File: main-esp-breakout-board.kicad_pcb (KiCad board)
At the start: 2 copper layers, 170.5 x 109 mm, 3 parts, among them J2 Conn_01x18_Pin, J3 Conn_01x18_Pin

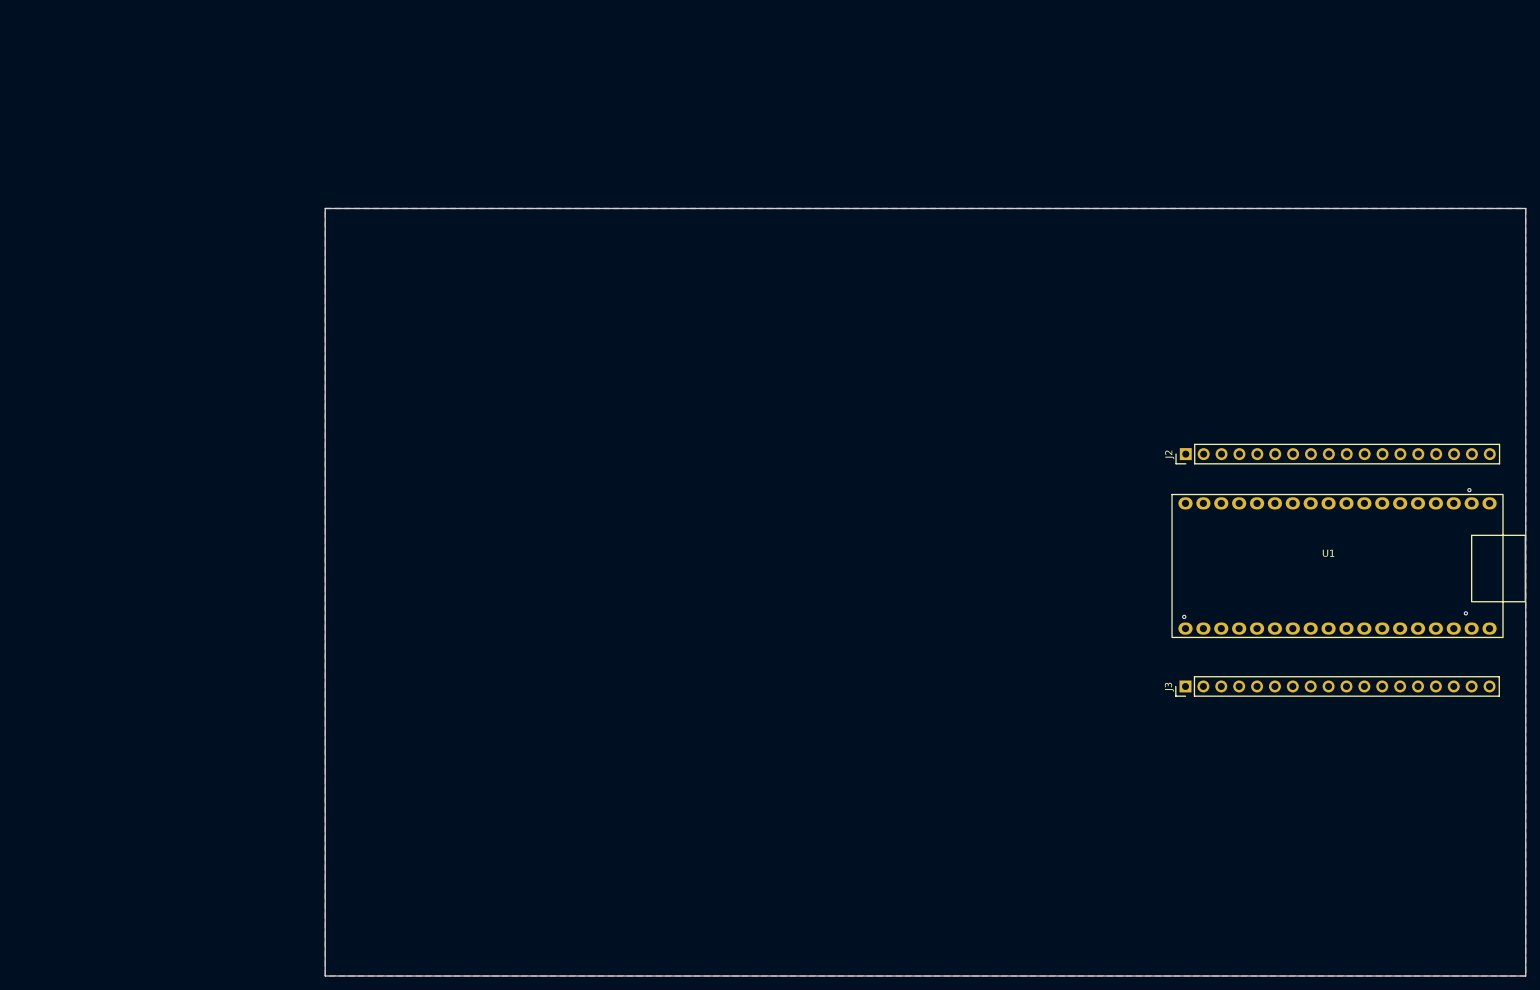
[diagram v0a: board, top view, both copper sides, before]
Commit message: halfway thru layout...
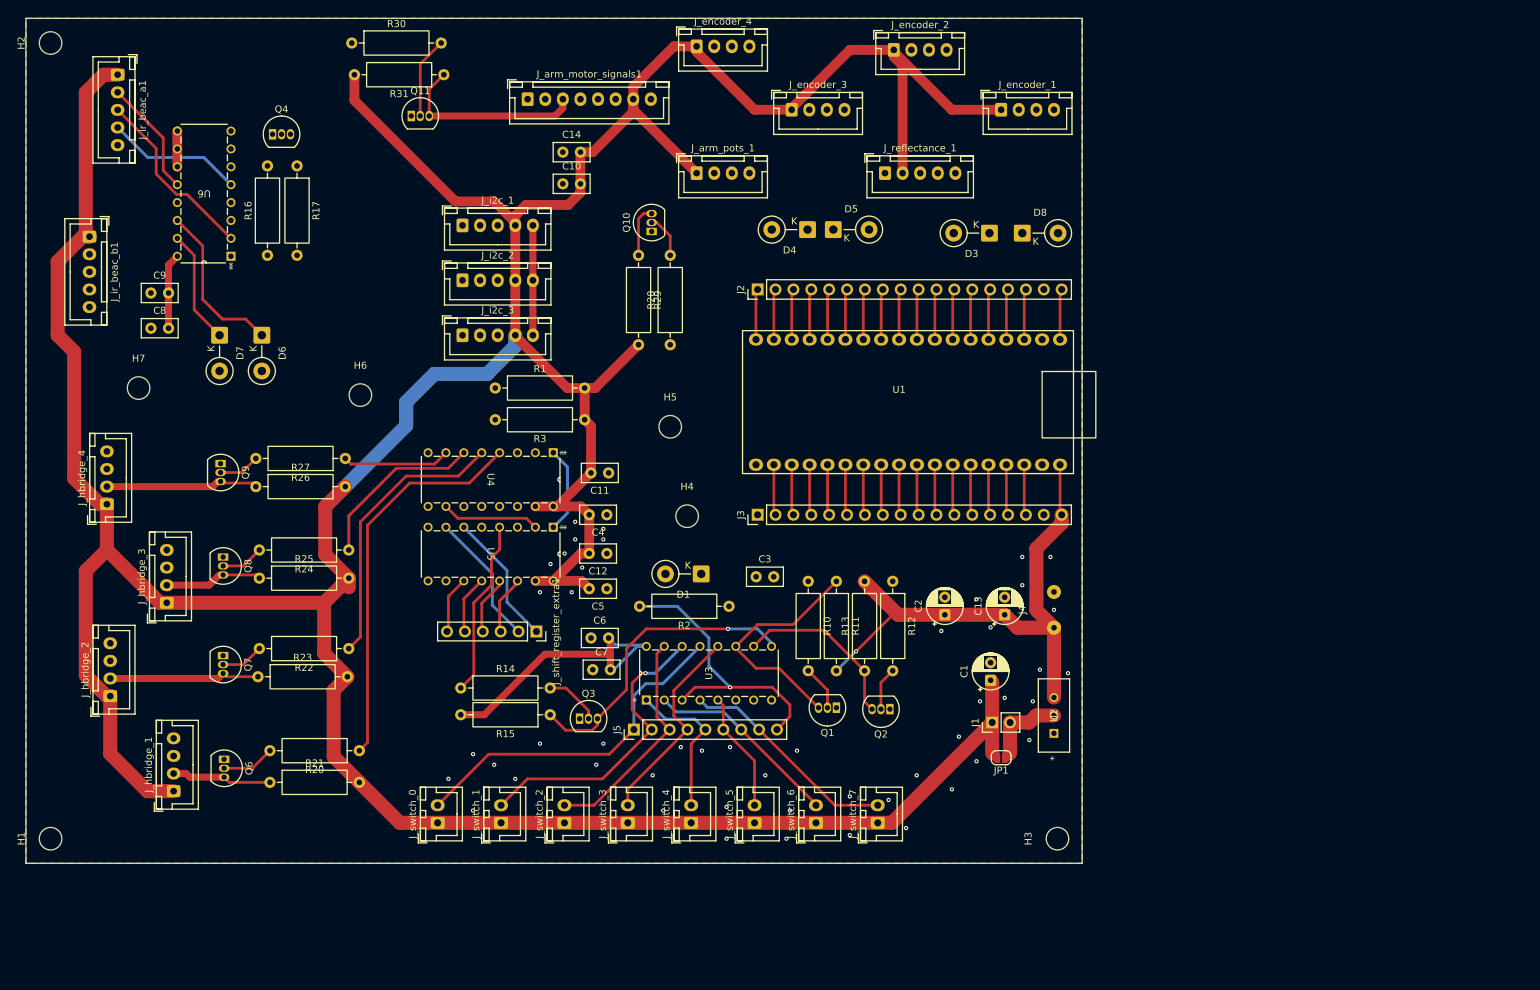
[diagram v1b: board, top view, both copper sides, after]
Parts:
- added C1: 10uf, Capacitor_THT:CP_Radial_D5.0mm_P2.50mm, F.Cu at (149.5, 106.5)
- added C10: 1nF, Capacitor_THT:C_Disc_D5.0mm_W2.5mm_P2.50mm, F.Cu at (88.8, 36.0)
- added C11: 1nF, Capacitor_THT:C_Disc_D5.0mm_W2.5mm_P2.50mm, F.Cu at (95.2, 77.1)
- added C12: 1nF, Capacitor_THT:C_Disc_D5.0mm_W2.5mm_P2.50mm, F.Cu at (95.0, 88.5)
- added C13: 10uf, Capacitor_THT:CP_Radial_D5.0mm_P2.50mm, F.Cu at (151.5, 97.2)
- added C14: 1nF, Capacitor_THT:C_Disc_D5.0mm_W2.5mm_P2.50mm, F.Cu at (88.8, 31.5)
- added C2: 1uf, Capacitor_THT:CP_Radial_D5.0mm_P2.50mm, F.Cu at (143.0, 97.2)
- added C3: 100nF, Capacitor_THT:C_Disc_D5.0mm_W2.5mm_P2.50mm, F.Cu at (116.2, 91.8)
- added C4: 1nF, Capacitor_THT:C_Disc_D5.0mm_W2.5mm_P2.50mm, F.Cu at (95.0, 83.0)
- added C5: 1nF, Capacitor_THT:C_Disc_D5.0mm_W2.5mm_P2.50mm, F.Cu at (95.0, 93.5)
- added C6: 1nF, Capacitor_THT:C_Disc_D5.0mm_W2.5mm_P2.50mm, F.Cu at (92.8, 100.5)
- added C7: 1nF, Capacitor_THT:C_Disc_D5.0mm_W2.5mm_P2.50mm, F.Cu at (93.0, 105.0)
- added C8: 1nF, Capacitor_THT:C_Disc_D5.0mm_W2.5mm_P2.50mm, F.Cu at (30.2, 56.5)
- added C9: 1nF, Capacitor_THT:C_Disc_D5.0mm_W2.5mm_P2.50mm, F.Cu at (30.2, 51.5)
- added D1: 3V3, Diode_THT:D_DO-15_P5.08mm_Vertical_KathodeUp, F.Cu at (108.4, 91.4)
- added D3: 3V3, Diode_THT:D_DO-15_P5.08mm_Vertical_KathodeUp, F.Cu at (149.3, 43.0)
- added D4: 3V3, Diode_THT:D_DO-15_P5.08mm_Vertical_KathodeUp, F.Cu at (123.5, 42.5)
- added D5: 3V3, Diode_THT:D_DO-15_P5.08mm_Vertical_KathodeUp, F.Cu at (127.2, 42.5)
- added D6: 3V3, Diode_THT:D_DO-15_P5.08mm_Vertical_KathodeUp, F.Cu at (46.0, 57.5)
- added D7: 3V3, Diode_THT:D_DO-15_P5.08mm_Vertical_KathodeUp, F.Cu at (40.0, 57.5)
- added D8: 3V3, Diode_THT:D_DO-15_P5.08mm_Vertical_KathodeUp, F.Cu at (154.0, 43.0)
- added H1: MountingHole, MountingHole:MountingHole_3.2mm_M3, F.Cu at (16.0, 129.0)
- added H2: MountingHole, MountingHole:MountingHole_3.2mm_M3, F.Cu at (16.0, 16.0)
- added H3: MountingHole, MountingHole:MountingHole_3.2mm_M3, F.Cu at (159.0, 129.0)
- added H4: MountingHole, MountingHole:MountingHole_3.2mm_M3, F.Cu at (106.4, 83.2)
- added H5: MountingHole, MountingHole:MountingHole_3.2mm_M3, F.Cu at (104.0, 70.5)
- added H6: MountingHole, MountingHole:MountingHole_3.2mm_M3, F.Cu at (60.0, 66.0)
- added H7: MountingHole, MountingHole:MountingHole_3.2mm_M3, F.Cu at (28.5, 65.0)
- added J1: Conn_01x02_Pin, Connector_PinHeader_2.54mm:PinHeader_1x02_P2.54mm_Vertical, F.Cu at (149.7, 112.5)
- added J4: Conn_01x02_Socket, Project_Lib:Power_Connector, F.Cu at (158.5, 96.5)
- added J5: Conn_01x09_Pin, Connector_PinHeader_2.54mm:PinHeader_1x09_P2.54mm_Vertical, F.Cu at (98.8, 113.5)
- added JP1: SolderJumper_2_Open, Jumper:SolderJumper-2_P1.3mm_Open_RoundedPad1.0x1.5mm, F.Cu at (151.0, 117.5)
- added J_arm_motor_signals1: Conn_01x08_Socket, Connector_JST:JST_XH_B8B-XH-A_1x08_P2.50mm_Vertical, F.Cu at (83.8, 24.0)
- added J_arm_pots_1: Conn_01x04_Socket, Connector_JST:JST_XH_B4B-XH-A_1x04_P2.50mm_Vertical, F.Cu at (107.8, 34.5)
- added J_encoder_1: Conn_01x04_Socket, Connector_JST:JST_XH_B4B-XH-A_1x04_P2.50mm_Vertical, F.Cu at (151.0, 25.5)
- added J_encoder_2: Conn_01x04_Socket, Connector_JST:JST_XH_B4B-XH-A_1x04_P2.50mm_Vertical, F.Cu at (135.8, 17.0)
- added J_encoder_3: Conn_01x04_Socket, Connector_JST:JST_XH_B4B-XH-A_1x04_P2.50mm_Vertical, F.Cu at (121.2, 25.5)
- added J_encoder_4: Conn_01x04_Socket, Connector_JST:JST_XH_B4B-XH-A_1x04_P2.50mm_Vertical, F.Cu at (107.8, 16.5)
- added J_hbridge_1: Conn_01x04_Socket, Connector_JST:JST_XH_B4B-XH-A_1x04_P2.50mm_Vertical, F.Cu at (33.5, 122.2)
- added J_hbridge_2: Conn_01x04_Socket, Connector_JST:JST_XH_B4B-XH-A_1x04_P2.50mm_Vertical, F.Cu at (24.5, 108.8)
- added J_hbridge_3: Conn_01x04_Socket, Connector_JST:JST_XH_B4B-XH-A_1x04_P2.50mm_Vertical, F.Cu at (32.5, 95.5)
- added J_hbridge_4: Conn_01x04_Socket, Connector_JST:JST_XH_B4B-XH-A_1x04_P2.50mm_Vertical, F.Cu at (24.0, 81.5)
- added J_i2c_1: Conn_01x05_Socket, Connector_JST:JST_XH_B5B-XH-A_1x05_P2.50mm_Vertical, F.Cu at (74.5, 41.9)
- added J_i2c_2: Conn_01x05_Socket, Connector_JST:JST_XH_B5B-XH-A_1x05_P2.50mm_Vertical, F.Cu at (74.5, 49.7)
- added J_i2c_3: Conn_01x05_Socket, Connector_JST:JST_XH_B5B-XH-A_1x05_P2.50mm_Vertical, F.Cu at (74.5, 57.5)
- added J_ir_beac_a1: Conn_01x05_Socket, Connector_JST:JST_XH_B5B-XH-A_1x05_P2.50mm_Vertical, F.Cu at (25.5, 20.5)
- added J_ir_beac_b1: Conn_01x05_Socket, Connector_JST:JST_XH_B5B-XH-A_1x05_P2.50mm_Vertical, F.Cu at (21.5, 43.5)
- added J_reflectance_1: Conn_01x05_Socket, Connector_JST:JST_XH_B5B-XH-A_1x05_P2.50mm_Vertical, F.Cu at (134.5, 34.5)
- added J_shift_register_extra1: Conn_01x06_Pin, Connector_PinSocket_2.54mm:PinSocket_1x06_P2.54mm_Vertical, F.Cu at (85.0, 99.6)
- added J_switch_0: Conn_01x02_Socket, Connector_JST:JST_XH_B2B-XH-A_1x02_P2.50mm_Vertical, F.Cu at (71.0, 126.8)
- added J_switch_1: Conn_01x02_Socket, Connector_JST:JST_XH_B2B-XH-A_1x02_P2.50mm_Vertical, F.Cu at (80.0, 126.8)
- added J_switch_2: Conn_01x02_Socket, Connector_JST:JST_XH_B2B-XH-A_1x02_P2.50mm_Vertical, F.Cu at (89.0, 126.8)
- added J_switch_3: Conn_01x02_Socket, Connector_JST:JST_XH_B2B-XH-A_1x02_P2.50mm_Vertical, F.Cu at (98.0, 126.8)
- added J_switch_4: Conn_01x02_Socket, Connector_JST:JST_XH_B2B-XH-A_1x02_P2.50mm_Vertical, F.Cu at (107.0, 126.8)
- added J_switch_5: Conn_01x02_Socket, Connector_JST:JST_XH_B2B-XH-A_1x02_P2.50mm_Vertical, F.Cu at (116.0, 126.8)
- added J_switch_6: Conn_01x02_Socket, Connector_JST:JST_XH_B2B-XH-A_1x02_P2.50mm_Vertical, F.Cu at (124.7, 126.8)
- added J_switch_7: Conn_01x02_Socket, Connector_JST:JST_XH_B2B-XH-A_1x02_P2.50mm_Vertical, F.Cu at (133.5, 126.8)
- added Q1: 2N3904, Package_TO_SOT_THT:TO-92_Inline, F.Cu at (127.6, 110.4)
- added Q10: 2N3904, Package_TO_SOT_THT:TO-92_Inline, F.Cu at (101.4, 42.8)
- added Q11: 2N3904, Package_TO_SOT_THT:TO-92_Inline, F.Cu at (67.2, 26.4)
- added Q2: 2N3904, Package_TO_SOT_THT:TO-92_Inline, F.Cu at (135.2, 110.6)
- added Q3: 2N3904, Package_TO_SOT_THT:TO-92_Inline, F.Cu at (91.1, 112.0)
- added Q4: 2N3904, Package_TO_SOT_THT:TO-92_Inline, F.Cu at (47.5, 29.0)
- added Q6: 2N3904, Package_TO_SOT_THT:TO-92_Inline, F.Cu at (40.6, 117.7)
- added Q7: 2N3904, Package_TO_SOT_THT:TO-92_Inline, F.Cu at (40.5, 103.0)
- added Q8: 2N3904, Package_TO_SOT_THT:TO-92_Inline, F.Cu at (40.5, 89.0)
- added Q9: 2N3904, Package_TO_SOT_THT:TO-92_Inline, F.Cu at (40.1, 75.7)
- added R1: 4.7k, Resistor_THT:R_Axial_DIN0309_L9.0mm_D3.2mm_P12.70mm_Horizontal, F.Cu at (79.2, 65.0)
- added R10: 100k, Resistor_THT:R_Axial_DIN0309_L9.0mm_D3.2mm_P12.70mm_Horizontal, F.Cu at (123.6, 92.5)
- added R11: 10k, Resistor_THT:R_Axial_DIN0309_L9.0mm_D3.2mm_P12.70mm_Horizontal, F.Cu at (127.6, 92.5)
- added R12: 100k, Resistor_THT:R_Axial_DIN0309_L9.0mm_D3.2mm_P12.70mm_Horizontal, F.Cu at (135.6, 92.5)
- added R13: 10k, Resistor_THT:R_Axial_DIN0309_L9.0mm_D3.2mm_P12.70mm_Horizontal, F.Cu at (131.6, 105.2)
- added R14: 100k, Resistor_THT:R_Axial_DIN0309_L9.0mm_D3.2mm_P12.70mm_Horizontal, F.Cu at (74.2, 107.6)
- added R15: 10k, Resistor_THT:R_Axial_DIN0309_L9.0mm_D3.2mm_P12.70mm_Horizontal, F.Cu at (87.0, 111.4)
- added R16: 100k, Resistor_THT:R_Axial_DIN0309_L9.0mm_D3.2mm_P12.70mm_Horizontal, F.Cu at (46.8, 46.1)
- added R17: 10k, Resistor_THT:R_Axial_DIN0309_L9.0mm_D3.2mm_P12.70mm_Horizontal, F.Cu at (51.0, 33.5)
- added R2: 4.7k, Resistor_THT:R_Axial_DIN0309_L9.0mm_D3.2mm_P12.70mm_Horizontal, F.Cu at (112.3, 96.0)
- added R20: 100k, Resistor_THT:R_Axial_DIN0309_L9.0mm_D3.2mm_P12.70mm_Horizontal, F.Cu at (59.9, 116.5)
- added R21: 10k, Resistor_THT:R_Axial_DIN0309_L9.0mm_D3.2mm_P12.70mm_Horizontal, F.Cu at (47.1, 121.0)
- added R22: 100k, Resistor_THT:R_Axial_DIN0309_L9.0mm_D3.2mm_P12.70mm_Horizontal, F.Cu at (58.4, 102.0)
- added R23: 10k, Resistor_THT:R_Axial_DIN0309_L9.0mm_D3.2mm_P12.70mm_Horizontal, F.Cu at (45.5, 106.0)
- added R24: 100k, Resistor_THT:R_Axial_DIN0309_L9.0mm_D3.2mm_P12.70mm_Horizontal, F.Cu at (58.4, 88.0)
- added R25: 10k, Resistor_THT:R_Axial_DIN0309_L9.0mm_D3.2mm_P12.70mm_Horizontal, F.Cu at (45.6, 92.0)
- added R26: 100k, Resistor_THT:R_Axial_DIN0309_L9.0mm_D3.2mm_P12.70mm_Horizontal, F.Cu at (57.9, 75.0)
- added R27: 10k, Resistor_THT:R_Axial_DIN0309_L9.0mm_D3.2mm_P12.70mm_Horizontal, F.Cu at (45.1, 79.0)
- added R28: 100k, Resistor_THT:R_Axial_DIN0309_L9.0mm_D3.2mm_P12.70mm_Horizontal, F.Cu at (104.0, 58.9)
- added R29: 10k, Resistor_THT:R_Axial_DIN0309_L9.0mm_D3.2mm_P12.70mm_Horizontal, F.Cu at (99.5, 46.1)
- added R3: 4.7k, Resistor_THT:R_Axial_DIN0309_L9.0mm_D3.2mm_P12.70mm_Horizontal, F.Cu at (91.8, 69.5)
- added R30: 100k, Resistor_THT:R_Axial_DIN0309_L9.0mm_D3.2mm_P12.70mm_Horizontal, F.Cu at (58.8, 16.0)
- added R31: 10k, Resistor_THT:R_Axial_DIN0309_L9.0mm_D3.2mm_P12.70mm_Horizontal, F.Cu at (71.8, 20.5)
- added U2: MC33269T-3.3, Project_Lib:TO220-3_ONS, F.Cu at (158.5, 114.0)
- added U3: CD4051B, Project_Lib:N16, F.Cu at (118.4, 101.7)
- added U4: CD74HC4094E, Project_Lib:N16, F.Cu at (69.6, 81.8)
- added U5: CD74HC4094E, Project_Lib:N16, F.Cu at (69.6, 92.4)
- added U6: CD4053B, Project_Lib:N16, F.Cu at (34.0, 28.5)
- moved J3 65.5 mm to (116.4, 83.0)
- moved U1 65.3 mm to (136.5, 65.7)
- moved J2 65.1 mm to (116.4, 51.0)
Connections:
- net +3.3V renamed esp_3.3
- J2 pad 11: 10 -> 1
- U1 pad 1: 10 -> 1
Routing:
- net supply_3.3: track 0.00 -> 600.9 mm
- net +5V: track 0.00 -> 145.5 mm, vias 0 -> 1
- net SHIFT_0: track 0.00 -> 55.5 mm
- net S_MUX_0: track 0.00 -> 49.4 mm
- net Net-(Q3-C): track 0.00 -> 43.6 mm, vias 0 -> 1
- net S_MUX_1: track 0.00 -> 42.9 mm, vias 0 -> 1
- net MUX_BYPASS: track 0.00 -> 41.3 mm, vias 0 -> 1
- net SHIFT_1: track 0.00 -> 40.0 mm
- net Net-(Q1-C): track 0.00 -> 34.0 mm
- net S_MUX_2: track 0.00 -> 32.4 mm
- net S_MUX_7: track 0.00 -> 31.4 mm
- net 35: track 0.00 -> 30.4 mm
- net S_MUX_3: track 0.00 -> 29.5 mm
- net S_MUX_6: track 0.00 -> 27.8 mm
- net Net-(J_arm_motor_signals1-Pin_3): track 0.00 -> 27.4 mm
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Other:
- board size 170.5 x 109 mm -> 150 x 120 mm
